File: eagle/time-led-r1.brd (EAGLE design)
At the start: 74.9 x 39.4 mm, 8 parts

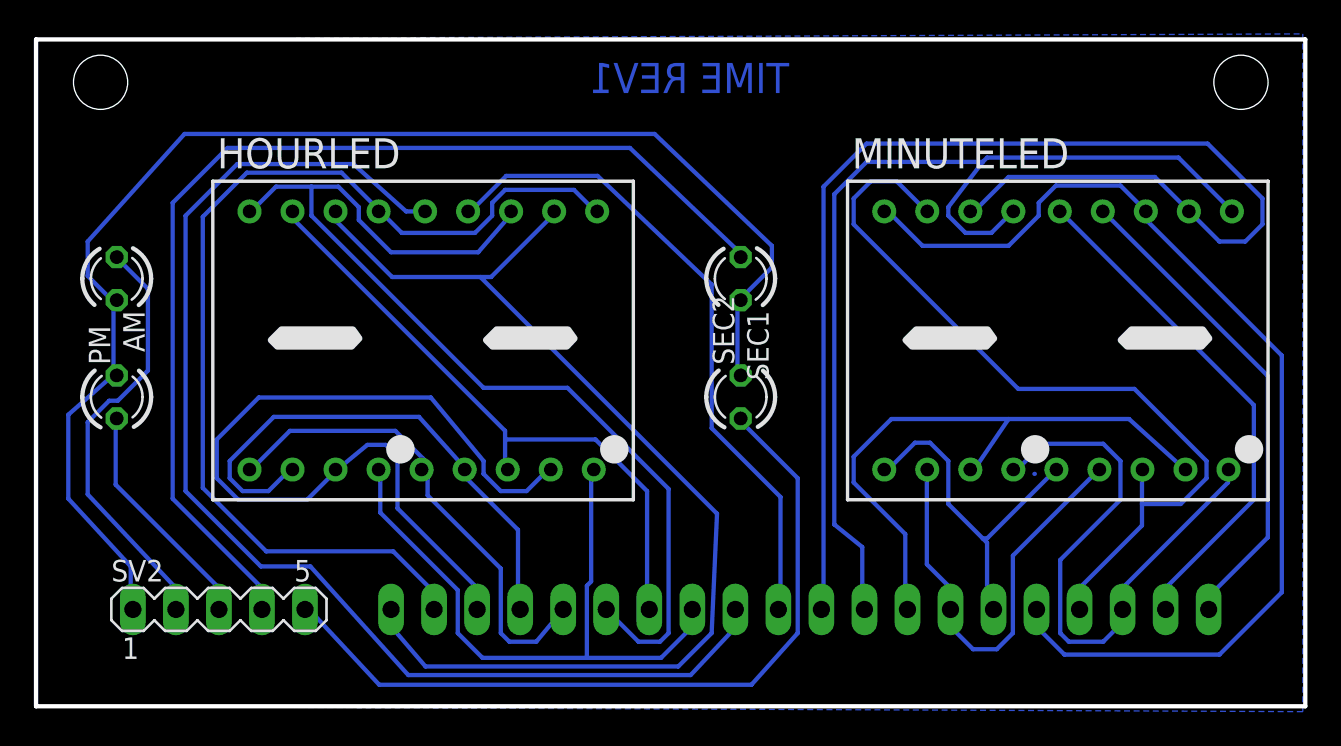
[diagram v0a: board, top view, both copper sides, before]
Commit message: More schematics
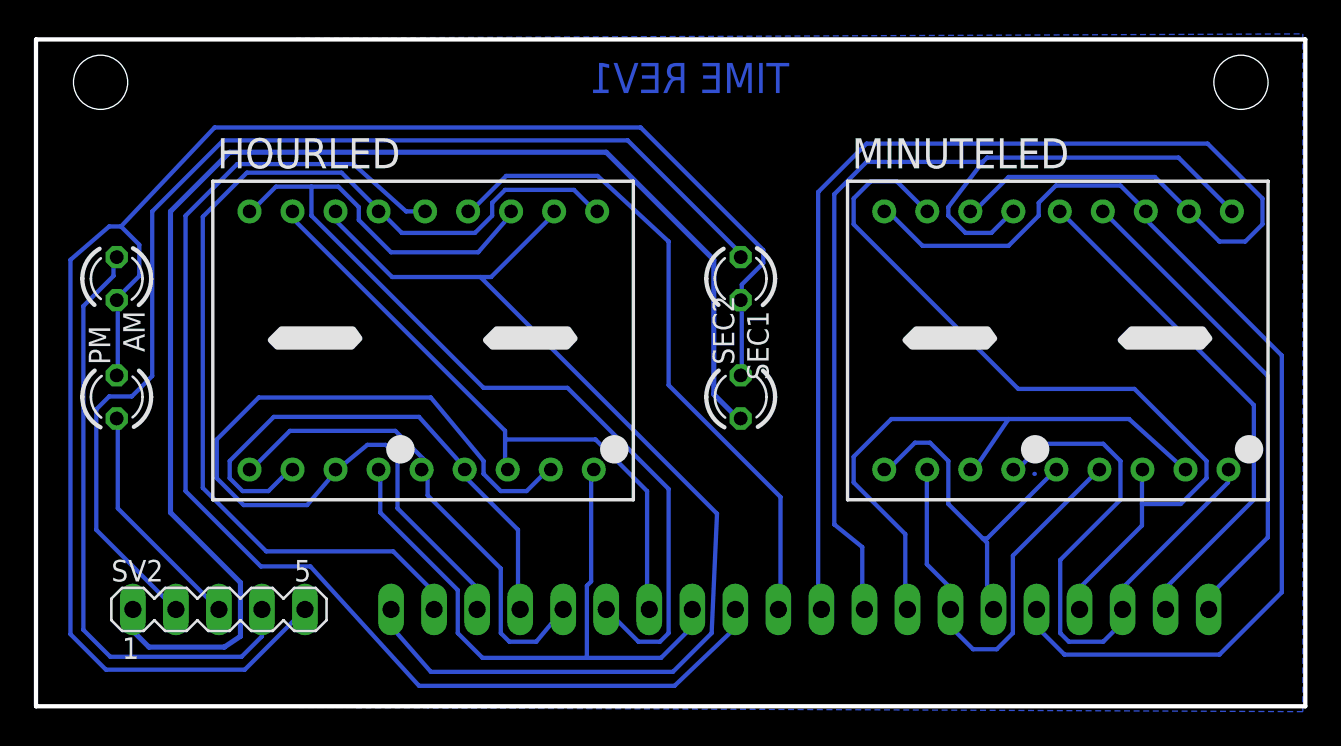
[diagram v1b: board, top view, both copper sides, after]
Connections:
- net N$19: now also SV2.5; no longer SV2.1
- net N$21: now also SV2.4; no longer SV2.2
- net N$23: now also SV2.2; no longer SV2.4
- net N$24: now also SV2.1; no longer SV2.5
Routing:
- net N$24: track 46.5 -> 81.6 mm
- net N$19: track 80.0 -> 103.3 mm
- net N$21: track 25.4 -> 36.1 mm
- net N$23: track 64.1 -> 67.4 mm
